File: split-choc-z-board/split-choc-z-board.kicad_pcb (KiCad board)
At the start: 2 copper layers, 122.3 x 98.6 mm, 45 parts, among them J1 USB4105-GF-A, SW1 SW_SPST, SW10 SW_SPST, SW11 SW_SPST, SW12 SW_SPST, SW13 SW_SPST, SW14 SW_SPST, SW15 SW_SPST, SW16 SW_SPST, SW17 SW_SPST, SW18 SW_SPST, SW2 SW_SPST, SW3 SW_SPST, SW4 SW_SPST, SW5 SW_SPST, SW6 SW_SPST, SW7 SW_SPST, SW8 SW_SPST, SW9 SW_SPST, U1 USBLC6-2SC6

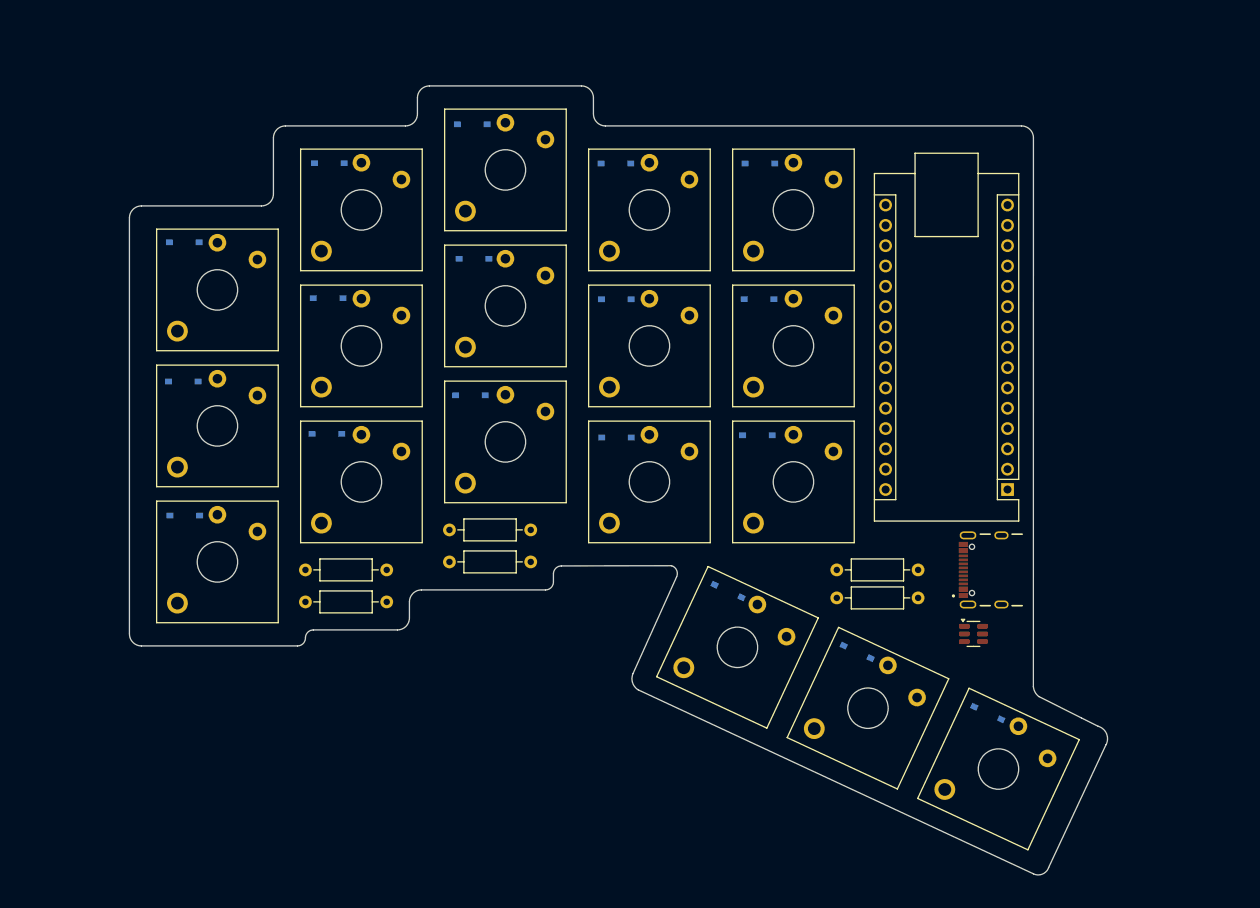
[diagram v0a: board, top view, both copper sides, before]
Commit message: Routed left side! 😃
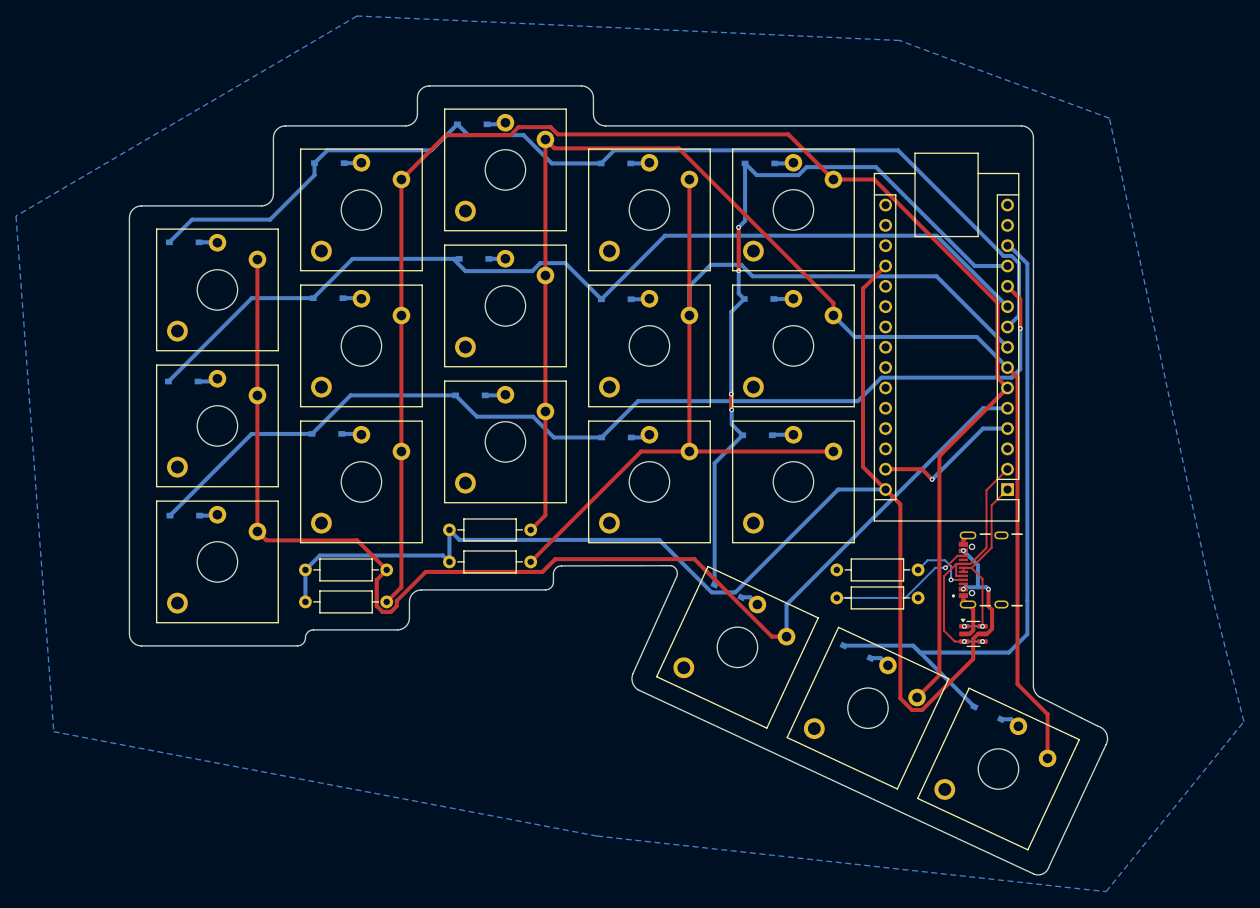
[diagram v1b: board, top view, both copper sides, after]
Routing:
- net /Column 2: track 0.00 -> 194.4 mm
- net +5V: track 0.00 -> 178.9 mm, vias 0 -> 3
- net /Column 3: track 0.00 -> 171.0 mm
- net /Column 1: track 0.00 -> 157.6 mm
- net /Row 1: track 0.00 -> 130.3 mm
- net /Row 3: track 0.00 -> 129.3 mm, vias 0 -> 1
- net /Column 4: track 0.00 -> 126.4 mm
- net /Row 2: track 0.00 -> 121.9 mm
- net /Row 4: track 0.00 -> 94.9 mm, vias 0 -> 4
- net /Row 5: track 0.00 -> 84.8 mm
- net /RX: track 0.00 -> 32.3 mm, vias 0 -> 2
- net GND: track 0.00 -> 25.9 mm, vias 0 -> 1
- net /TX: track 0.00 -> 23.3 mm, vias 0 -> 2
- net /CC2: track 0.00 -> 18.1 mm, vias 0 -> 1
- net /CC1: track 0.00 -> 8.17 mm, vias 0 -> 1
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- added copper zone on B.Cu, net GND
